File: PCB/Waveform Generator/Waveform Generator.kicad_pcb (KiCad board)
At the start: 4 copper layers, 141 parts, among them J1 Power input, J10 USART1_2, J11 5001, J12 Signal 2, J13 5001, J14 5001, J15 5001, J16 5001, J17 5001, J18 5001, J19 ADC_2, J2 RS485_1, J20 TIMER_1, J21 I2C1_1, J22 TIMER_2, J23 I2C1_2, J3 USB_B_Micro, J4 5001, J5 Signal 1, J6 SWD, J7 RS485_2, J8 USART1_1, J9 ADC_1, Q0 AO3401A, Q1 Q_NPN_BCE, Q2 Q_NPN_BCE, Q3 Q_PNP_BCE, Q4 Q_NPN_BCE, Q5 Q_NPN_BCE, Q6 Q_NPN_BCE, Q7 Q_NPN_BCE, Q8 Q_NPN_BCE, SW1 SW_SPDT, SW2 RESET Button, SW3 SW_SPDT, SW4 Btn1, SW5 Btn1, SW6 Btn1, SW7 SW_SPDT, U1 STM32F427VITx, U10 USBLC6-2SC6, U11 USBLC6-2SC6, U2 MAX485EESAT, U3 USBLC6-2SC6, U4 OPA1602, U5 OPA1602, U6 USBLC6-2SC6, U7 USBLC6-2SC6, U8 LM335ADT, U9 USBLC6-2SC6, X1 25MHZ

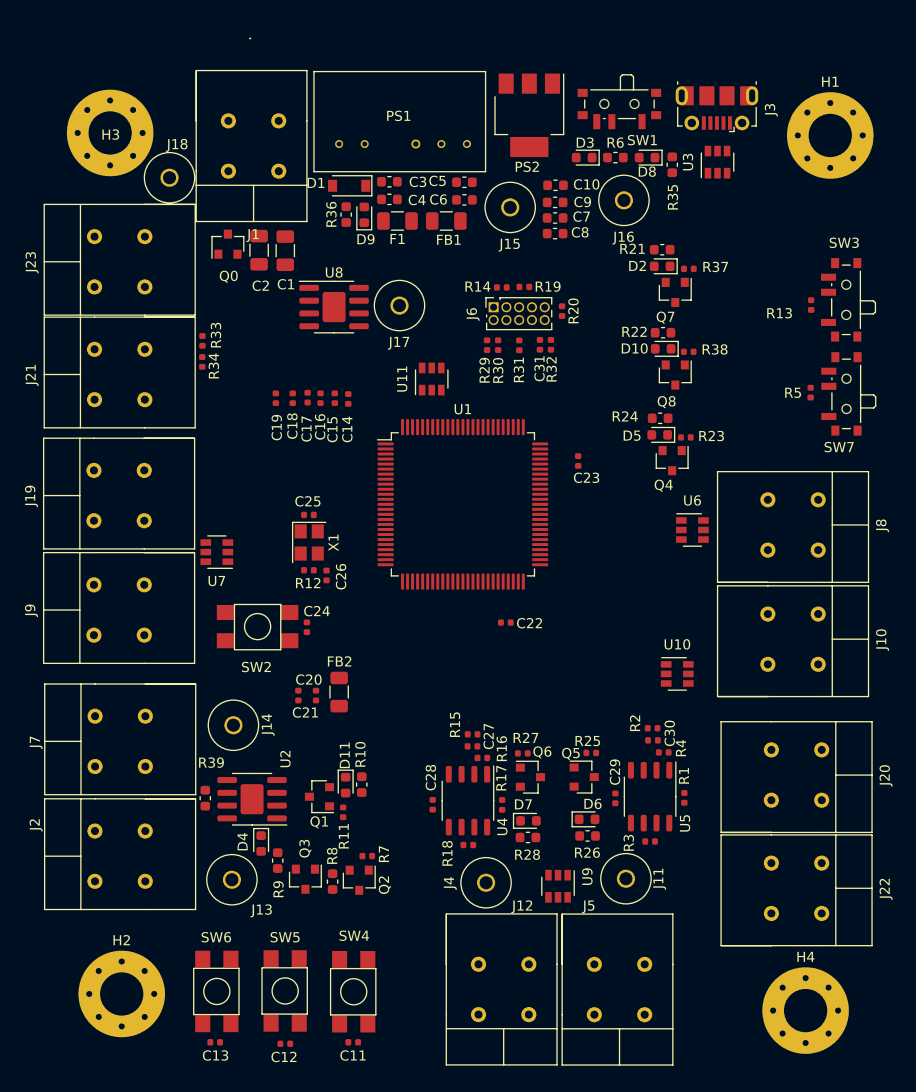
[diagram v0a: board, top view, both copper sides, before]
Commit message: Making good progress
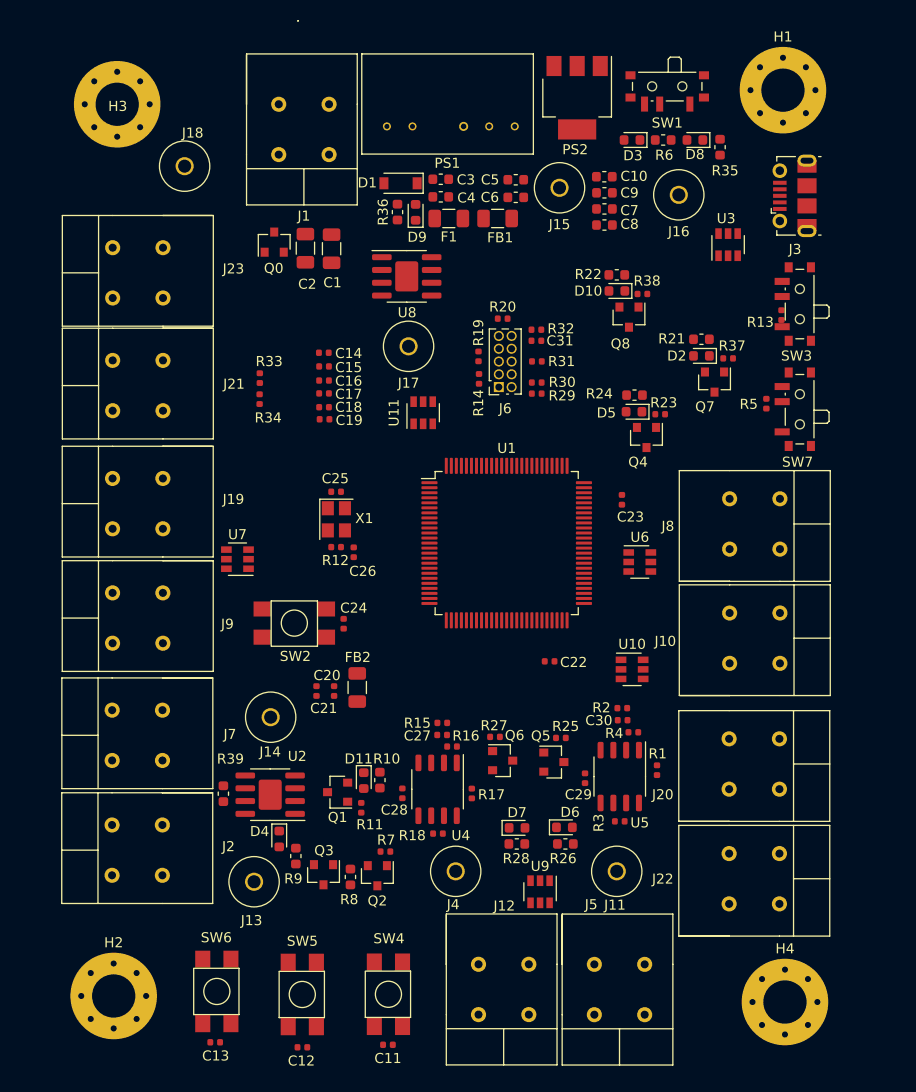
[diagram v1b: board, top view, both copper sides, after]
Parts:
- moved J3 11.6 mm to (89.8, 25.9), turned to 90 degrees
- moved R37 9.72 mm to (83.2, 42.0)
- moved R21 9.72 mm to (80.5, 40.1)
- moved D2 9.72 mm to (80.5, 41.8)
- moved Q7 9.72 mm to (81.8, 44.4)
- moved R14 9.36 mm to (58.5, 44.0), turned to 270 degrees
- moved U3 8.27 mm to (83.2, 30.7)
- moved R19 8.27 mm to (58.4, 41.8), turned to 90 degrees
- moved J6 7.95 mm to (60.4, 44.9), turned to 180 degrees
- moved U8 7.84 mm to (51.3, 33.9)
- moved Q8 7.36 mm to (73.3, 37.9)
- moved D10 7.36 mm to (72.2, 35.3)
- moved R22 7.36 mm to (72.1, 33.7)
- moved R38 7.36 mm to (74.7, 35.6)
- moved R29 6.89 mm to (64.2, 45.5), turned to 180 degrees
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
